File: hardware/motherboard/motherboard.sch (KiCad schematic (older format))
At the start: 21 parts, among them J1 DB37_Female, J10 DB37_Female, J11 DB37_Female, J12 Barrel_Jack, J13 TSR 1-2433, J2 DB37_Female, J3 DB37_Female, J4 DB37_Female, J5 DB37_Female, J6 DB25_Female, J7 DB37_Female, J8 DB25_Female, J9 DB9_Female, SW1 SW_SPST

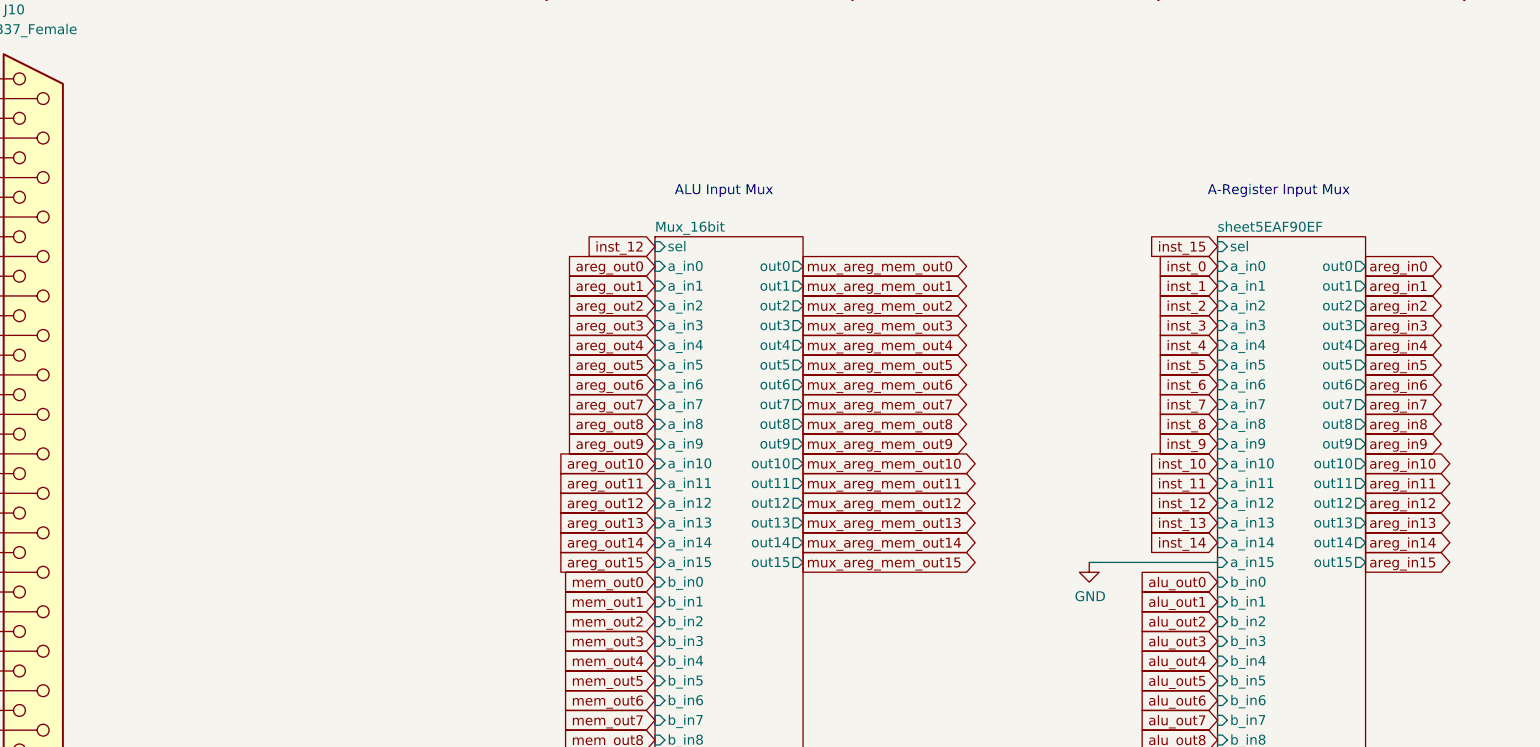
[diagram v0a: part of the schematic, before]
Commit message: All boards as fabbed at v1.0
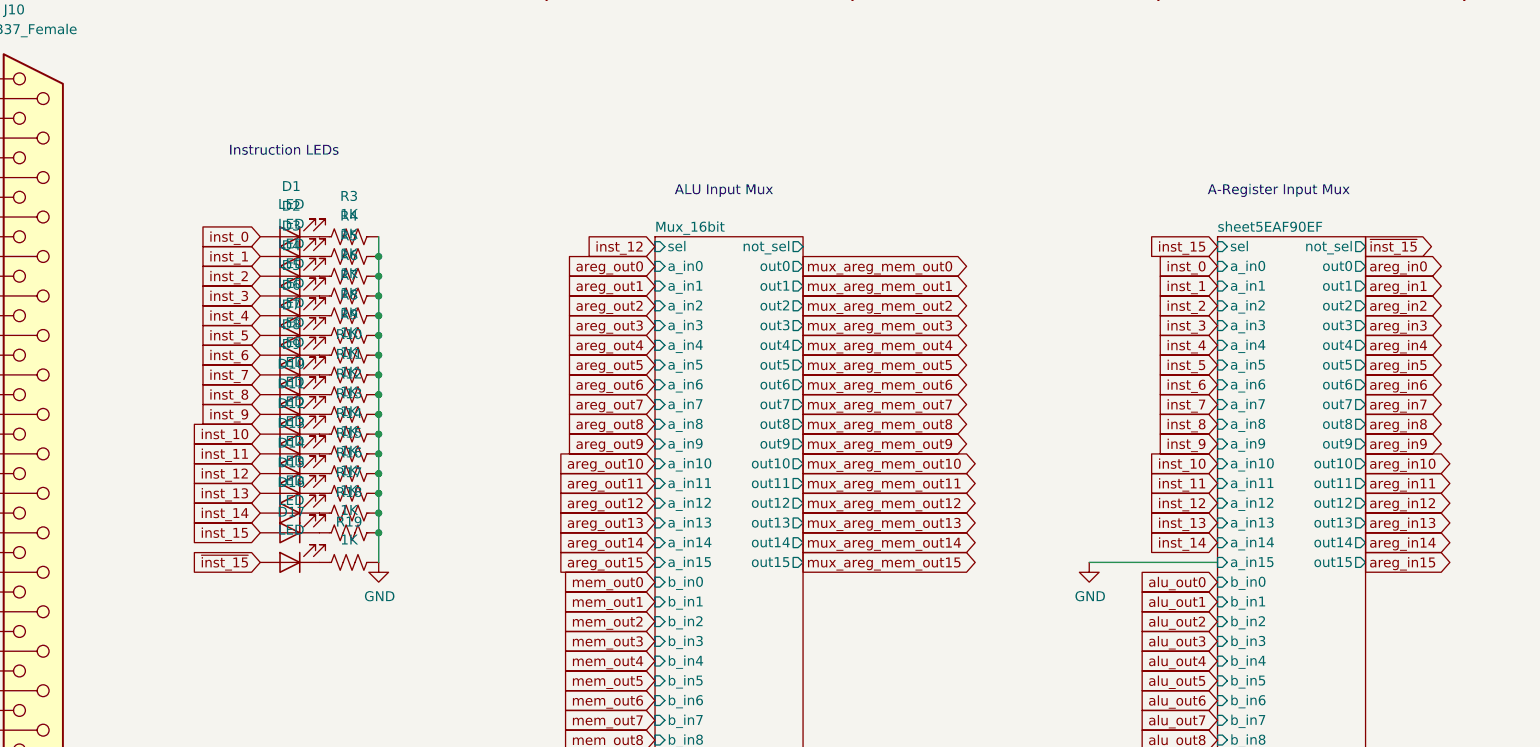
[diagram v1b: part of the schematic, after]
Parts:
- added D1, D10, D11, D12, D13, D14, D15, D16, D17, D2, D3, D4, D5, D6, D7, D8, D9: LED, LED_SMD:LED_1206_3216Metric, symbol Device:LED
- added R10, R11, R12, R13, R14, R15, R16, R17, R18, R19, R3, R4, R5, R6, R7, R8, R9: 1K, Resistor_SMD:R_1206_3216Metric, symbol Device:R_US
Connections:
- net GND: now also R10.1, R11.1, R12.1, R13.1, R14.1, R15.1, R16.1, R17.1, R18.1, R19.1, R3.1, R4.1, R5.1, R6.1, R7.1, R8.1, R9.1
- net inst_0: now also D1.2 (A)
- net inst_1: now also D2.2 (A)
- net inst_10: now also D11.2 (A)
- net inst_11: now also D12.2 (A)
- net inst_12: now also D13.2 (A)
- net inst_13: now also D14.2 (A)
- net inst_14: now also D15.2 (A)
- net inst_15: now also D16.2 (A)
- net inst_2: now also D3.2 (A)
- net inst_3: now also D4.2 (A)
- net inst_4: now also D5.2 (A)
- net inst_5: now also D6.2 (A)
- net inst_6: now also D7.2 (A)
- net inst_7: now also D8.2 (A)
- net inst_8: now also D9.2 (A)
- net inst_9: now also D10.2 (A)
- new net: D1.1 (K), R3.2
- new net: D2.1 (K), R4.2
- new net: D3.1 (K), R5.2
- new net: D4.1 (K), R6.2
- new net: D5.1 (K), R7.2
- new net: D6.1 (K), R8.2
- new net: D7.1 (K), R9.2
- new net: D8.1 (K), R10.2
- new net: D9.1 (K), R11.2
- new net: D10.1 (K), R12.2
- new net: D11.1 (K), R13.2
- new net: D12.1 (K), R14.2
- new net: D13.1 (K), R15.2
- new net: D14.1 (K), R16.2
- new net: D15.1 (K), R17.2
- new net: D16.1 (K), R18.2
- new net: D17.1 (K), R19.2
- new net ~inst_15: D17.2 (A)
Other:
- note added: "Instruction LEDs"
